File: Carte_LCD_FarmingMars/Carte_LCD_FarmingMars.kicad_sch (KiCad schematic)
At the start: 21 parts, among them J2 Conn_01x02_Pin, J3 Conn_01x04_Pin, J4 Conn_01x02_Pin, SW1 SW_DIP_x01, SW2 SW_Push, SW3 SW_Push, U1 3V3 reg, U2 ATtiny1616-S

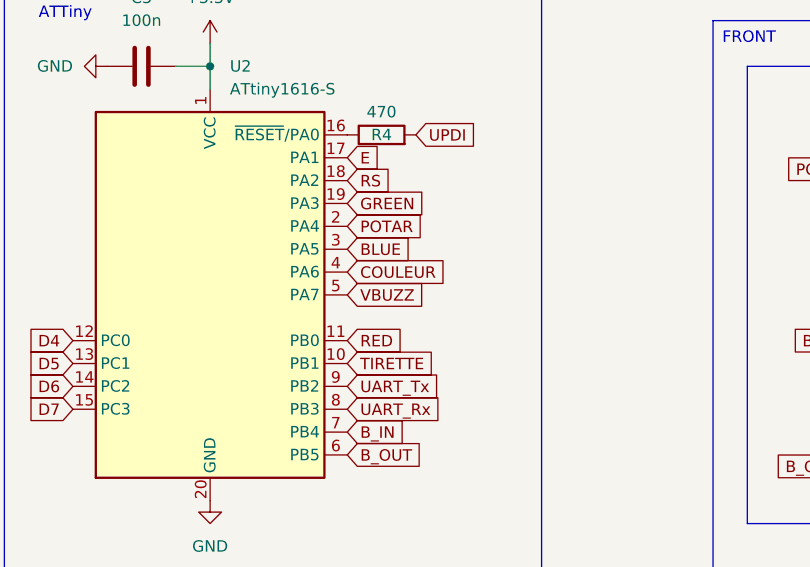
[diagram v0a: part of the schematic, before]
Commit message: Routage, inversion pin Couleur et Vbuzz
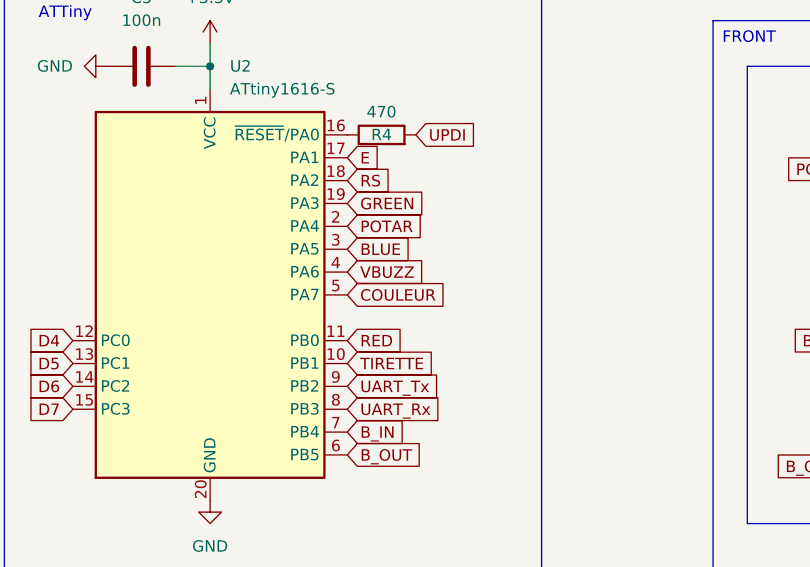
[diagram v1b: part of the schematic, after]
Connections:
- net COULEUR: now also U2.5 (PA7); no longer U2.4 (PA6)
- net VBUZZ: now also U2.4 (PA6); no longer U2.5 (PA7)
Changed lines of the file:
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@@
     )
   )
-  (global_label "COULEUR" (shape input) (at 58.42 110.49 0) (fields_autoplaced)
+  (global_label "COULEUR" (shape input) (at 58.42 113.03 0) (fields_autoplaced)
     (effects (font (size 1.27 1.27)) (justify left))
-    (property "Intersheetrefs" "${INTERSHEET_REFS}" (at 70.1138 110.49 0)
+    (property "Intersheetrefs" "${INTERSHEET_REFS}" (at 70.1138 113.03 0)
       (effects (font (size 1.27 1.27)) (justify left) hide)
     )
@@
     )
   )
-  (global_label "VBUZZ" (shape input) (at 58.42 113.03 0) (fields_autoplaced)
+  (global_label "VBUZZ" (shape input) (at 58.42 110.49 0) (fields_autoplaced)
     (effects (font (size 1.27 1.27)) (justify left))
-    (property "Intersheetrefs" "${INTERSHEET_REFS}" (at 67.5133 113.03 0)
+    (property "Intersheetrefs" "${INTERSHEET_REFS}" (at 67.5133 110.49 0)
       (effects (font (size 1.27 1.27)) (justify left) hide)
     )
